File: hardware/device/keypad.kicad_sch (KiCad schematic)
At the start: 76 parts, among them SW1 TRIG1, SW10 TRIG10, SW11 TRIG11, SW12 TRIG12, SW13 TRIG13, SW14 TRIG14, SW15 TRIG15, SW16 TRIG16, SW17 WHEEL_BTN, SW18 HELP, SW19 LEFT_BTN, SW2 TRIG2, SW20 RIGHT_BTN, SW3 TRIG3, SW4 TRIG4, SW5 TRIG5, SW6 TRIG6, SW7 TRIG7, SW8 TRIG8, SW9 TRIG9, U25 TCA8418RTWR

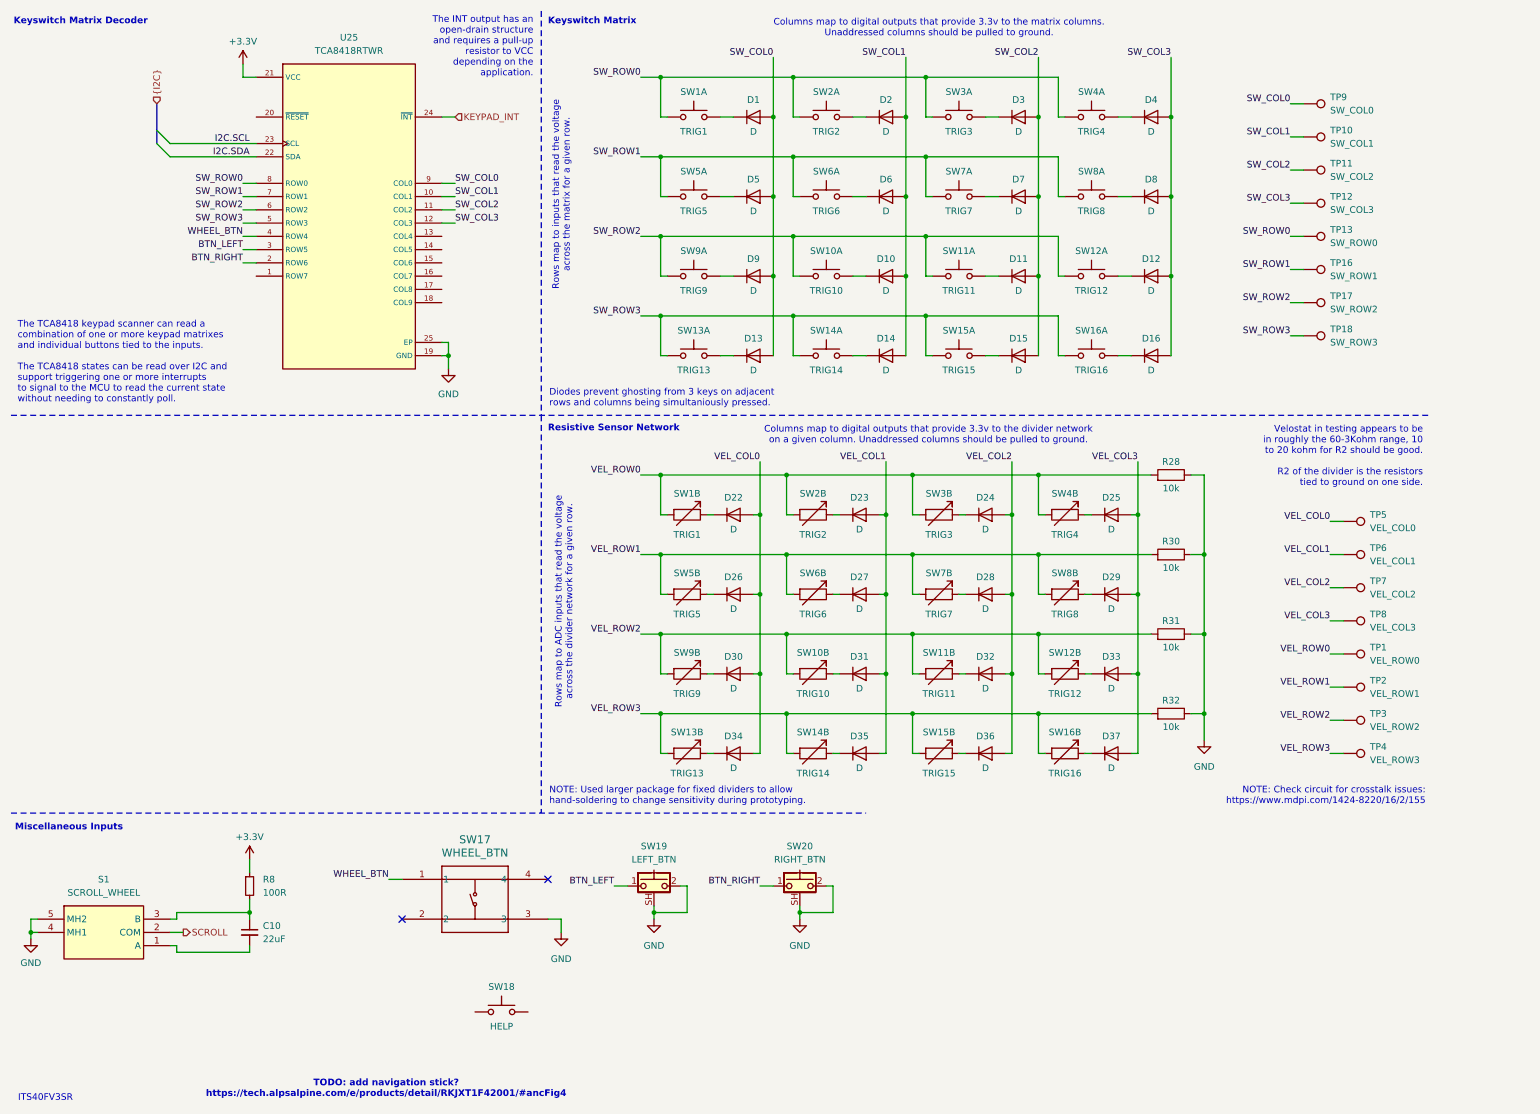
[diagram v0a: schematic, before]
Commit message: chore: schematic organization
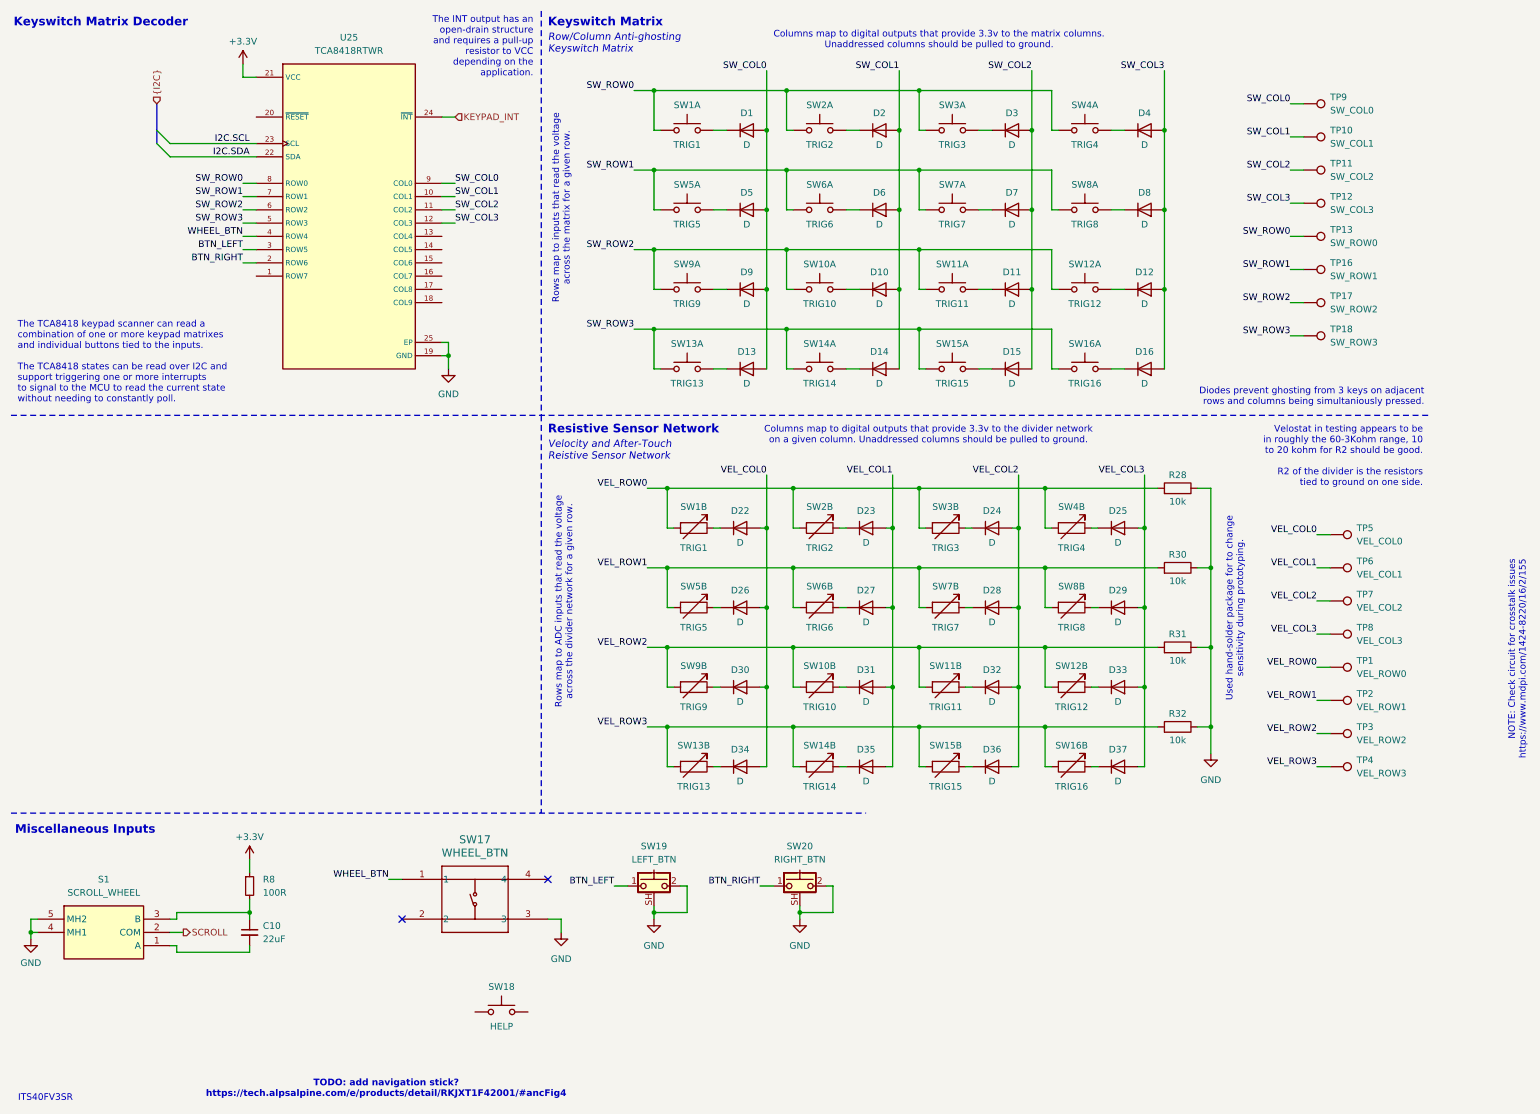
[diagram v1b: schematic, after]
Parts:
- C10: footprint (none) -> Capacitor_SMD:C_0402_1005Metric
- R8: footprint (none) -> Resistor_SMD:R_0402_1005Metric
- TP1, TP10, TP11, TP12, TP13, TP16, TP17, TP18, TP2, TP3, TP4, TP5, TP6, TP7, TP8, TP9: footprint TestPoint:TestPoint_Pad_D2.5mm -> TestPoint:TestPoint_Pad_D1.5mm
- U25: JLC (none) -> C138713
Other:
- note added: "NOTE: Check circuit for crosstalk issues https://www.mdpi.com/1424-8220/16/2/155"
- note added: "Row/Column Anti-ghosting Keyswitch Matrix"
- note added: "Used hand-solder package for to change sensitivity during prototyping."
- note added: "Velocity and After-Touch Reistive Sensor Network"
- note removed: "NOTE: Check circuit for crosstalk issues: https://www.mdpi.com/1424-8220/16/2/155"
- note removed: "NOTE: Used larger package for fixed dividers to allow hand-soldering to change sensitivity during prototyping."
- moved on the sheet: D1, D10, D11, D12, D13, D14, D15, D16, D2, D22, D23, D24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
